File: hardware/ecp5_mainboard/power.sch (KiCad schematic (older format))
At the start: 103 parts, among them J1 12V_EXT, Q1 BSH111BKR, Q2 BC850, Q3 BSH111BKR, Q4 BC850, Q5 BSH111BKR, Q6 BSH111BKR, Q7 BSH111BKR, Q8 BSH111BKR, U1 MAX811MEUS-T, U10 TPS62823, U2 LM3880, U3 TLV75712PDR, U4 TPS565208, U5 LM21212-2, U6 TLV75712PDR, U7 TPS62823, U8 TPS62823, U9 TPS62823

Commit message: hardware/mainboard: Assign some footprints
Signed-off-by: David Shah <dave@ds0.me>
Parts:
- C1, C10: footprint (none) -> Capacitor_SMD:C_0603_1608Metric
- C11, C12, C19, C20, C21, C22, C7, C9: footprint (none) -> Capacitor_SMD:C_0402_1005Metric
- C13: footprint (none) -> Capacitor_SMD:C_1210_3225Metric
- C14, C15, C16, C17, C18, C23, C24, C25, C26, C27, C28, C29, C3, C30, C4, C5, C8: footprint (none) -> Capacitor_SMD:C_0805_2012Metric
- C6: footprint 22u/25V -> Capacitor_SMD:C_1206_3216Metric
- D1, D10, D11, D2, D4, D5, D6, D7, D8, D9: footprint (none) -> LED_SMD:LED_0805_2012Metric
- R1, R10, R11, R12, R13, R14, R15, R16, R17, R18, R19, R2, R20, R21, R22, R23, R24, R25, R26, R27, R28, R29, R3, R30, R31, R32, R33, R4, R5, R6, R7, R8, R9: footprint (none) -> Resistor_SMD:R_0402_1005Metric
- RN1: footprint (none) -> Resistor_SMD:R_Array_Convex_4x0402
- U4: footprint (none) -> Package_TO_SOT_SMD:SOT-23-6
- U5: footprint (none) -> Package_SO:HTSSOP-20-1EP_4.4x6.5mm_P0.65mm_EP3.4x6.5mm

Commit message: hardware/mainboard: Assign more footprints
Signed-off-by: David Shah <dave@ds0.me>
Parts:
- C2: footprint (none) -> Capacitor_SMD:CP_Elec_6.3x5.8
- J1: footprint (none) -> Connector_BarrelJack:BarrelJack_Horizontal
- L1: footprint (none) -> Inductor_SMD:L_Coilcraft_XAL5030
- L3, L4, L5, L6: footprint (none) -> Inductor_SMD:L_Vishay_IHLP-1212
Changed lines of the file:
@@
 F 0 "J1" H 1478 2975 50  0000 C CNN
 F 1 "12V_EXT" H 1478 2884 50  0000 C CNN
-F 2 "" H 1450 2610 50  0001 C CNN
+F 2 "Connector_BarrelJack:BarrelJack_Horizontal" H 1450 2610 50  0001 C CNN
 F 3 "~" H 1450 2610 50  0001 C CNN
 	1    1400 2650
@@
 F 0 "C2" H 3968 2746 50  0000 L CNN
 F 1 "100µF/25V" H 3968 2655 50  0000 L CNN
-F 2 "" H 3888 2550 50  0001 C CNN
+F 2 "Capacitor_SMD:CP_Elec_6.3x5.8" H 3888 2550 50  0001 C CNN
 F 3 "~" H 3850 2700 50  0001 C CNN
 	1    3850 2700
@@
 F 0 "L4" V 12340 1750 50  0000 C CNN
 F 1 "470n/IHLP1212" V 12249 1750 50  0000 C CNN
-F 2 "" H 12150 1750 50  0001 C CNN
+F 2 "Inductor_SMD:L_Vishay_IHLP-1212" H 12150 1750 50  0001 C CNN
 F 3 "~" H 12150 1750 50  0001 C CNN
 	1    12150 1750
@@
 F 0 "L5" V 12340 3250 50  0000 C CNN
 F 1 "470n/IHLP1212" V 12249 3250 50  0000 C CNN
-F 2 "" H 12150 3250 50  0001 C CNN
+F 2 "Inductor_SMD:L_Vishay_IHLP-1212" H 12150 3250 50  0001 C CNN
 F 3 "~" H 12150 3250 50  0001 C CNN
 	1    12150 3250
@@
 F 0 "L6" V 12340 4800 50  0000 C CNN
 F 1 "470n/IHLP1212" V 12249 4800 50  0000 C CNN
-F 2 "" H 12150 4800 50  0001 C CNN
+F 2 "Inductor_SMD:L_Vishay_IHLP-1212" H 12150 4800 50  0001 C CNN
 F 3 "~" H 12150 4800 50  0001 C CNN
 	1    12150 4800
@@
 F 0 "L3" V 12290 6250 50  0000 C CNN
 F 1 "470n/IHLP1212" V 12199 6250 50  0000 C CNN
-F 2 "" H 12100 6250 50  0001 C CNN
+F 2 "Inductor_SMD:L_Vishay_IHLP-1212" H 12100 6250 50  0001 C CNN
 F 3 "~" H 12100 6250 50  0001 C CNN
 	1    12100 6250
@@
 F 0 "L1" V 7590 6200 50  0000 C CNN
 F 1 "800nH/XAL5030" V 7499 6200 50  0000 C CNN
-F 2 "" H 7400 6200 50  0001 C CNN
+F 2 "Inductor_SMD:L_Coilcraft_XAL5030" H 7400 6200 50  0001 C CNN
 F 3 "~" H 7400 6200 50  0001 C CNN
 	1    7400 6200

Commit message: hardware: Creating and assigning some misc footprints
Signed-off-by: David Shah <dave@ds0.me>
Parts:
- F1, F2: footprint (none) -> Custom Parts:FuseHolder_SMD_Shurter_0031.7701.11
- L2: footprint (none) -> Custom Parts:L_CoilCraft_XAL60xx
- U3, U6: footprint (none) -> Custom Parts:TI_WSON8_2x2mm_p0.65mm
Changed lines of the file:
@@
 F 0 "F2" V 1953 2550 50  0000 C CNN
 F 1 "3A" V 2044 2550 50  0000 C CNN
-F 2 "" V 2080 2550 50  0001 C CNN
+F 2 "Custom Parts:FuseHolder_SMD_Shurter_0031.7701.11" V 2080 2550 50  0001 C CNN
 F 3 "~" H 2150 2550 50  0001 C CNN
 	1    2150 2550
@@
 F 0 "F1" V 1853 3600 50  0000 C CNN
 F 1 "3A/DNF" V 1944 3600 50  0000 C CNN
-F 2 "" V 1980 3600 50  0001 C CNN
+F 2 "Custom Parts:FuseHolder_SMD_Shurter_0031.7701.11" V 1980 3600 50  0001 C CNN
 F 3 "~" H 2050 3600 50  0001 C CNN
 	1    2050 3600
@@
 F 0 "L2" V 7690 2200 50  0000 C CNN
 F 1 "3.3µH/XAL6030-332" V 7599 2200 50  0000 C CNN
-F 2 "" H 7500 2200 50  0001 C CNN
+F 2 "Custom Parts:L_CoilCraft_XAL60xx" H 7500 2200 50  0001 C CNN
 F 3 "~" H 7500 2200 50  0001 C CNN
 	1    7500 2200
@@
 F 0 "U3" H 4100 10315 50  0000 C CNN
 F 1 "TLV75712PDR" H 4100 10224 50  0000 C CNN
-F 2 "" H 4100 9850 50  0001 C CNN
+F 2 "Custom Parts:TI_WSON8_2x2mm_p0.65mm" H 4100 9850 50  0001 C CNN
 F 3 "" H 4100 9850 50  0001 C CNN
 	1    4100 9850
@@
 F 0 "U6" H 8850 10365 50  0000 C CNN
 F 1 "TLV75712PDR" H 8850 10274 50  0000 C CNN
-F 2 "" H 8850 9900 50  0001 C CNN
+F 2 "Custom Parts:TI_WSON8_2x2mm_p0.65mm" H 8850 9900 50  0001 C CNN
 F 3 "" H 8850 9900 50  0001 C CNN
 	1    8850 9900

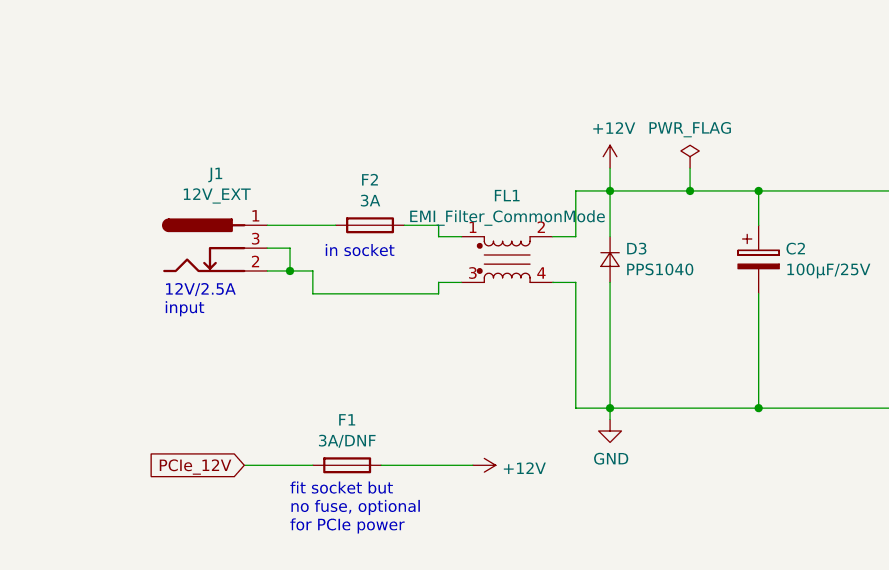
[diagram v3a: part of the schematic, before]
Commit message: hardware/mainboard: More footprint assignment, other small tweaks
Signed-off-by: David Shah <dave@ds0.me>
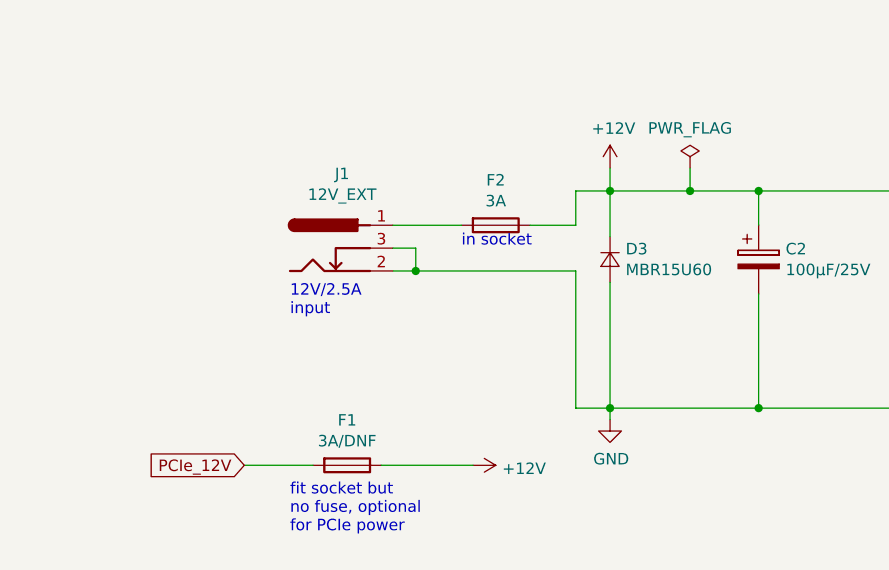
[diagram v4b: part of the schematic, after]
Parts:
- removed FL1: EMI_Filter_CommonMode, symbol Device:EMI_Filter_CommonMode
- D3: value PPS1040 -> MBR15U60
- U10, U7, U8, U9: footprint (none) -> Custom Parts:TI_VSON-HR_1.5x2mm_p0.5mm
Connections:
- net +12V: now also F2.1
- net GND: now also J1.2, J1.3
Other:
- moved on the sheet: F2, J1
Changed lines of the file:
@@
 L ecp5_mainboard-rescue:Barrel_Jack-Connector J1
 U 1 1 5B5D9C9C
-P 1400 2650
-F 0 "J1" H 1478 2975 50  0000 C CNN
-F 1 "12V_EXT" H 1478 2884 50  0000 C CNN
-F 2 "Connector_BarrelJack:BarrelJack_Horizontal" H 1450 2610 50  0001 C CNN
-F 3 "~" H 1450 2610 50  0001 C CNN
-	1    1400 2650
+P 1950 2650
+F 0 "J1" H 2028 2975 50  0000 C CNN
+F 1 "12V_EXT" H 2028 2884 50  0000 C CNN
+F 2 "Connector_BarrelJack:BarrelJack_Horizontal" H 2000 2610 50  0001 C CNN
+F 3 "~" H 2000 2610 50  0001 C CNN
+	1    1950 2650
 	1    0    0    -1
 $EndComp
@@
 L Device:Fuse F2
 U 1 1 5B5DA0F9
-P 2150 2550
-F 0 "F2" V 1953 2550 50  0000 C CNN
-F 1 "3A" V 2044 2550 50  0000 C CNN
-F 2 "Custom Parts:FuseHolder_SMD_Shurter_0031.7701.11" V 2080 2550 50  0001 C CNN
-F 3 "~" H 2150 2550 50  0001 C CNN
-	1    2150 2550
+P 2700 2550
+F 0 "F2" V 2503 2550 50  0000 C CNN
+F 1 "3A" V 2594 2550 50  0000 C CNN
+F 2 "Custom Parts:FuseHolder_SMD_Shurter_0031.7701.11" V 2630 2550 50  0001 C CNN
+F 3 "~" H 2700 2550 50  0001 C CNN
+	1    2700 2550
 	0    1    1    0
 $EndComp
 Wire Wire Line
-	1700 2550 2000 2550
-Wire Wire Line
-	1700 2750 1800 2750
-Wire Wire Line
-	1900 2750 1900 2850
-$Comp
-L Device:EMI_Filter_CommonMode FL1
-U 1 1 5B5DA3C4
-P 2750 2700
-F 0 "FL1" H 2750 2978 50  0000 C CNN
-F 1 "EMI_Filter_CommonMode" H 2750 2887 50  0000 C CNN
-F 2 "" V 2750 2740 50  0001 C CNN
-F 3 "~" V 2750 2740 50  0000 C CNN
-	1    2750 2700
-	1    0    0    -1
-$EndComp
-Wire Wire Line
-	2300 2550 2450 2550
-Wire Wire Line
-	2450 2550 2450 2600
-Wire Wire Line
-	2450 2600 2550 2600
-Wire Wire Line
-	2550 2800 2450 2800
-Wire Wire Line
-	2450 2800 2450 2850
-Wire Wire Line
-	1900 2850 2450 2850
-Wire Wire Line
-	2950 2800 3050 2800
-Wire Wire Line
-	3050 2800 3050 3350
+	2250 2550 2550 2550
+Wire Wire Line
+	2250 2750 2350 2750
 Wire Wire Line
 	3050 3350 3200 3350
-Wire Wire Line
-	2950 2600 3050 2600
-Wire Wire Line
-	3050 2600 3050 2400
 Wire Wire Line
 	3050 2400 3200 2400
@@
 P 3200 2700
 F 0 "D3" V 3154 2768 50  0000 L CNN
-F 1 "PPS1040" V 3245 2768 50  0000 L CNN
+F 1 "MBR15U60" V 3245 2768 50  0000 L CNN
 F 2 "" V 3200 2700 50  0001 C CNN
 F 3 "~" V 3200 2700 50  0001 C CNN
@@
 	3200 2800 3200 3350
 Wire Wire Line
-	1700 2650 1800 2650
-Wire Wire Line
-	1800 2650 1800 2750
-Connection ~ 1800 2750
-Wire Wire Line
-	1800 2750 1900 2750
+	2250 2650 2350 2650
+Wire Wire Line
+	2350 2650 2350 2750
+Connection ~ 2350 2750
 Connection ~ 3200 3350
 $Comp
@@
 Wire Wire Line
 	2200 3600 2600 3600
-Text Notes 1950 2700 0    50   ~ 0
+Text Notes 2550 2650 0    50   ~ 0
 in socket
 Text Notes 1800 3900 0    50   ~ 0
@@
 Wire Wire Line
 	8050 2150 8050 2200
-Text Notes 1250 2950 0    50   ~ 0
+Text Notes 1800 2950 0    50   ~ 0
 12V/2.5A\ninput
 $Comp
@@
 F 0 "U8" H 11150 2615 50  0000 C CNN
 F 1 "TPS62823" H 11150 2524 50  0000 C CNN
-F 2 "" H 11150 2050 50  0001 C CNN
+F 2 "Custom Parts:TI_VSON-HR_1.5x2mm_p0.5mm" H 11150 2050 50  0001 C CNN
 F 3 "http://www.ti.com/lit/ds/symlink/tps62823.pdf" H 11150 2050 50  0001 C CNN
 	1    11150 2050
@@
 F 0 "U9" H 11150 4115 50  0000 C CNN
 F 1 "TPS62823" H 11150 4024 50  0000 C CNN
-F 2 "" H 11150 3550 50  0001 C CNN
+F 2 "Custom Parts:TI_VSON-HR_1.5x2mm_p0.5mm" H 11150 3550 50  0001 C CNN
 F 3 "http://www.ti.com/lit/ds/symlink/tps62823.pdf" H 11150 3550 50  0001 C CNN
 	1    11150 3550
@@
 F 0 "U10" H 11150 5665 50  0000 C CNN
 F 1 "TPS62823" H 11150 5574 50  0000 C CNN
-F 2 "" H 11150 5100 50  0001 C CNN
+F 2 "Custom Parts:TI_VSON-HR_1.5x2mm_p0.5mm" H 11150 5100 50  0001 C CNN
 F 3 "http://www.ti.com/lit/ds/symlink/tps62823.pdf" H 11150 5100 50  0001 C CNN
 	1    11150 5100
@@
 F 0 "U7" H 11100 7115 50  0000 C CNN
 F 1 "TPS62823" H 11100 7024 50  0000 C CNN
-F 2 "" H 11100 6550 50  0001 C CNN
+F 2 "Custom Parts:TI_VSON-HR_1.5x2mm_p0.5mm" H 11100 6550 50  0001 C CNN
 F 3 "http://www.ti.com/lit/ds/symlink/tps62823.pdf" H 11100 6550 50  0001 C CNN
 	1    11100 6550
@@
 	8500 2150 8500 2200
 Connection ~ 8500 2200
+Wire Wire Line
+	3050 2750 3050 3350
+Wire Wire Line
+	2350 2750 3050 2750
+Wire Wire Line
+	3050 2550 3050 2400
+Wire Wire Line
+	2850 2550 3050 2550
 $EndSCHEMATC
